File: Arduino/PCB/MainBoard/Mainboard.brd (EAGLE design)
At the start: 94.9 x 80 mm, 62 parts, among them IC1 ULN2803ADW, IC2 DS1338Z-33+, J1 ARDUINO PROG, J2 BOOTL PROG, J3 DC-005, J4 XBEE CONN, Q1 32.768kHz, U1 ATMEGA328-AU, U4 R-78B5.0-2.0, X1 16Mhz

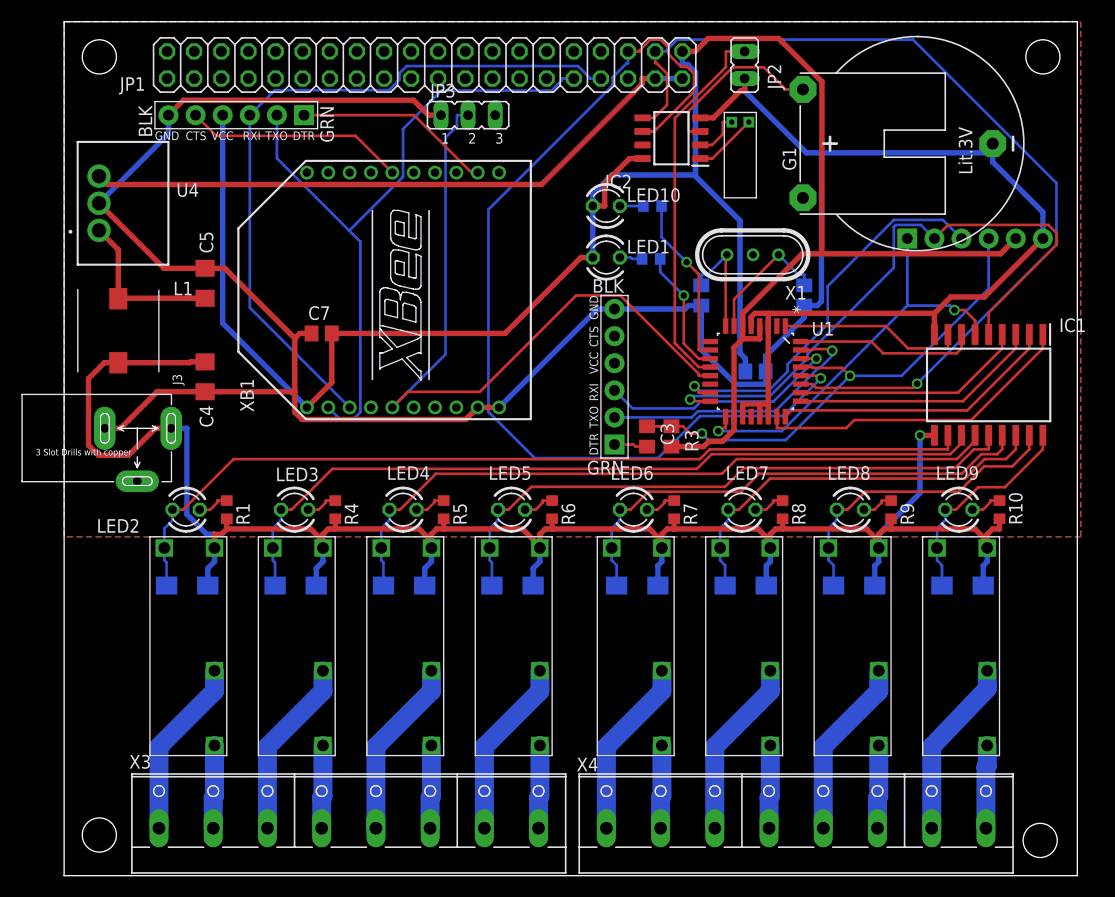
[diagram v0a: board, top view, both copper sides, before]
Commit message: as send to allpcb
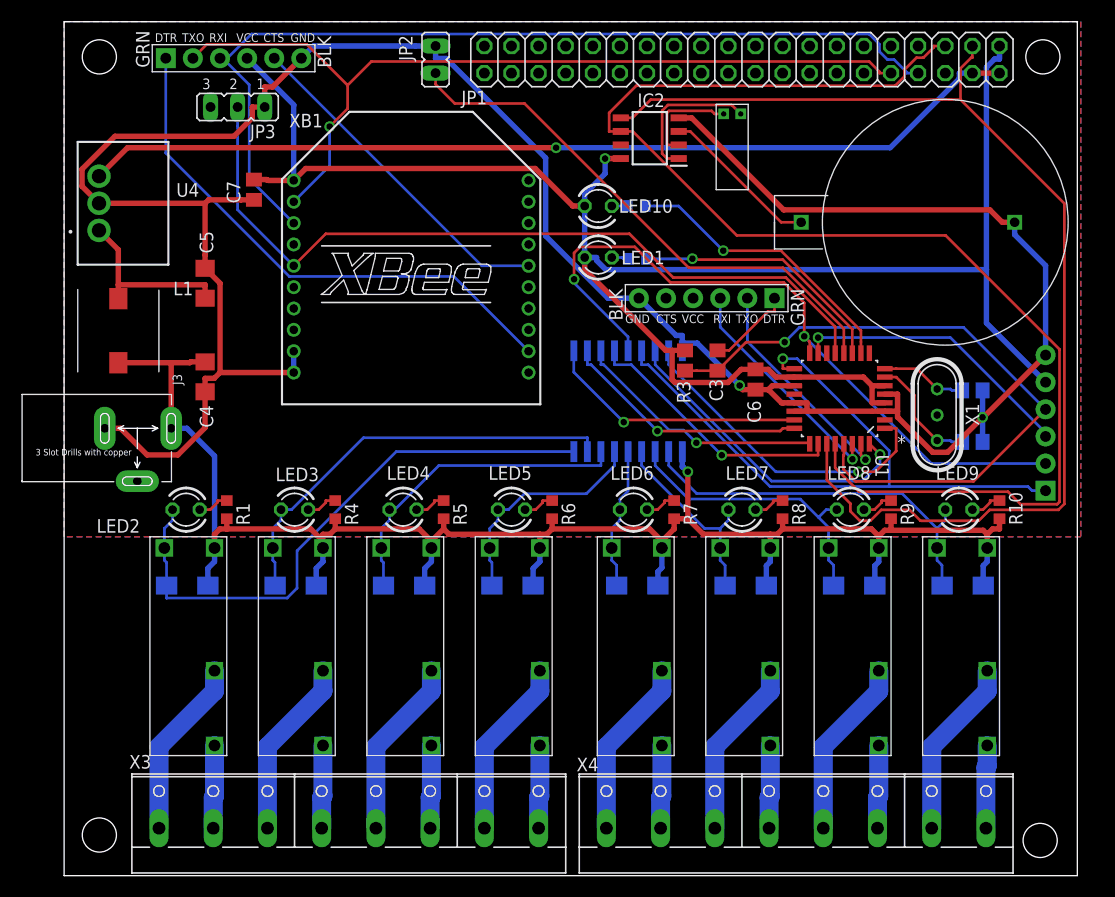
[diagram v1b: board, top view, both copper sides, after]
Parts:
- removed G1: CR2032, MainboardComponents:BATTERY_CR2032H
- added U$1: KEYSTONE_1066, MainboardComponents:KEYSTONE1066
- moved IC1 33.8 mm to (57.9, 44.5), flipped to the bottom
- moved JP1 29.7 mm to (68.6, 76.5)
- moved JP2 29.0 mm to (39.9, 76.5), turned to 180 degrees
- moved C1 26.9 mm to (90.2, 45.5), turned to 180 degrees
- moved X1 22.9 mm to (86.9, 43.2), turned to 90 degrees
- moved JP3 21.6 mm to (21.3, 72.0), turned to 180 degrees
- moved C2 20.9 mm to (90.2, 40.6), turned to 0 degrees
- moved J2 18.5 mm to (97.0, 42.4), turned to 90 degrees
- moved C7 14.9 mm to (22.9, 64.3), turned to 90 degrees
- moved J1 11.4 mm to (65.3, 54.1), turned to 180 degrees
- moved C3 9.71 mm to (66.3, 48.3), turned to 90 degrees
- moved U1 8.27 mm to (77.7, 44.7), turned to 180 degrees
- moved R3 7.22 mm to (63.2, 48.3), turned to 90 degrees
- moved J4 5.34 mm to (21.0, 76.6), turned to 0 degrees
- moved IC2 2.03 mm to (59.9, 69.1)
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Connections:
- net GND: now also U$1.NEG$2; no longer G1.-
- net N$12: now also U$1.POS$1; no longer G1.+
- net R0: now also DF1.A, LED2.K, REL0.A2; no longer DF8.A, LED9.K, REL7.A2
- net R1: now also DF2.A, LED3.K, REL1.A2; no longer DF7.A, LED8.K, REL6.A2
- net R2: now also DF3.A, LED4.K, REL2.A2; no longer DF6.A, LED7.K, REL5.A2
- net R3: now also DF4.A, LED5.K, REL3.A2; no longer DF5.A, LED6.K, REL4.A2
- net R4: now also DF5.A, LED6.K, REL4.A2; no longer DF4.A, LED5.K, REL3.A2
- net R5: now also DF6.A, LED7.K, REL5.A2; no longer DF3.A, LED4.K, REL2.A2
- net R6: now also DF7.A, LED8.K, REL6.A2; no longer DF2.A, LED3.K, REL1.A2
- net R7: now also DF8.A, LED9.K, REL7.A2; no longer DF1.A, LED2.K, REL0.A2
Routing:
- net R7: track 83.8 -> 36.5 mm
- net R6: track 74.6 -> 27.6 mm
- net R5: track 65.6 -> 18.7 mm
- net R4: track 57.1 -> 13.4 mm
- net R0: track 20.4 -> 54.6 mm
- net SCL: track 93.7 -> 126.0 mm, vias 1 -> 0
- net +3V3: track 203.1 -> 170.9 mm, vias 0 -> 1
- net N$13: track 18.5 -> 50.6 mm
- net +5V: track 59.4 -> 88.7 mm, vias 0 -> 1
- net R3: track 47.1 -> 21.5 mm
- net D5: track 39.0 -> 62.9 mm, vias 2 -> 1
- net +12V: track 181.1 -> 159.4 mm
- net SDA: track 87.5 -> 109.1 mm, vias 1 -> 0
- net N$35: track 67.0 -> 86.4 mm
- net N$3: track 64.4 -> 82.0 mm, vias 0 -> 1
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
